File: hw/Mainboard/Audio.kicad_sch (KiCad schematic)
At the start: 10 parts, among them J1 SJ-43504-SMT-TR, J8 SPEAKER, Q2 MMBT3904

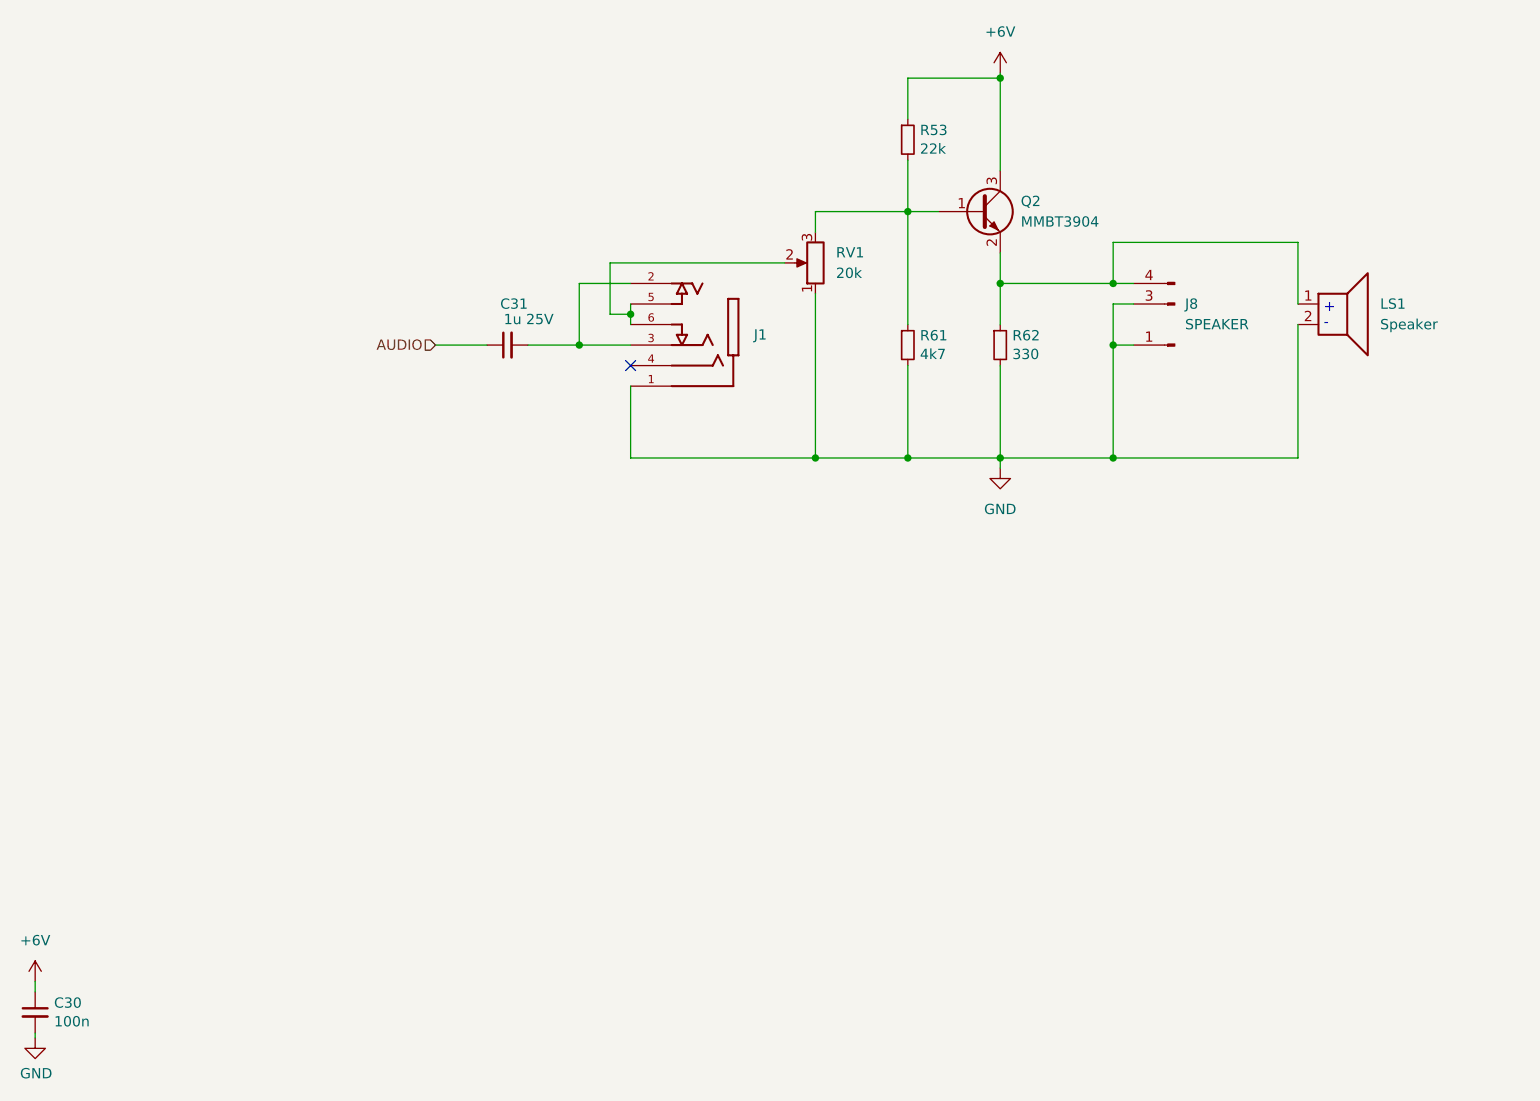
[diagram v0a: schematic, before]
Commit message: hw: wip
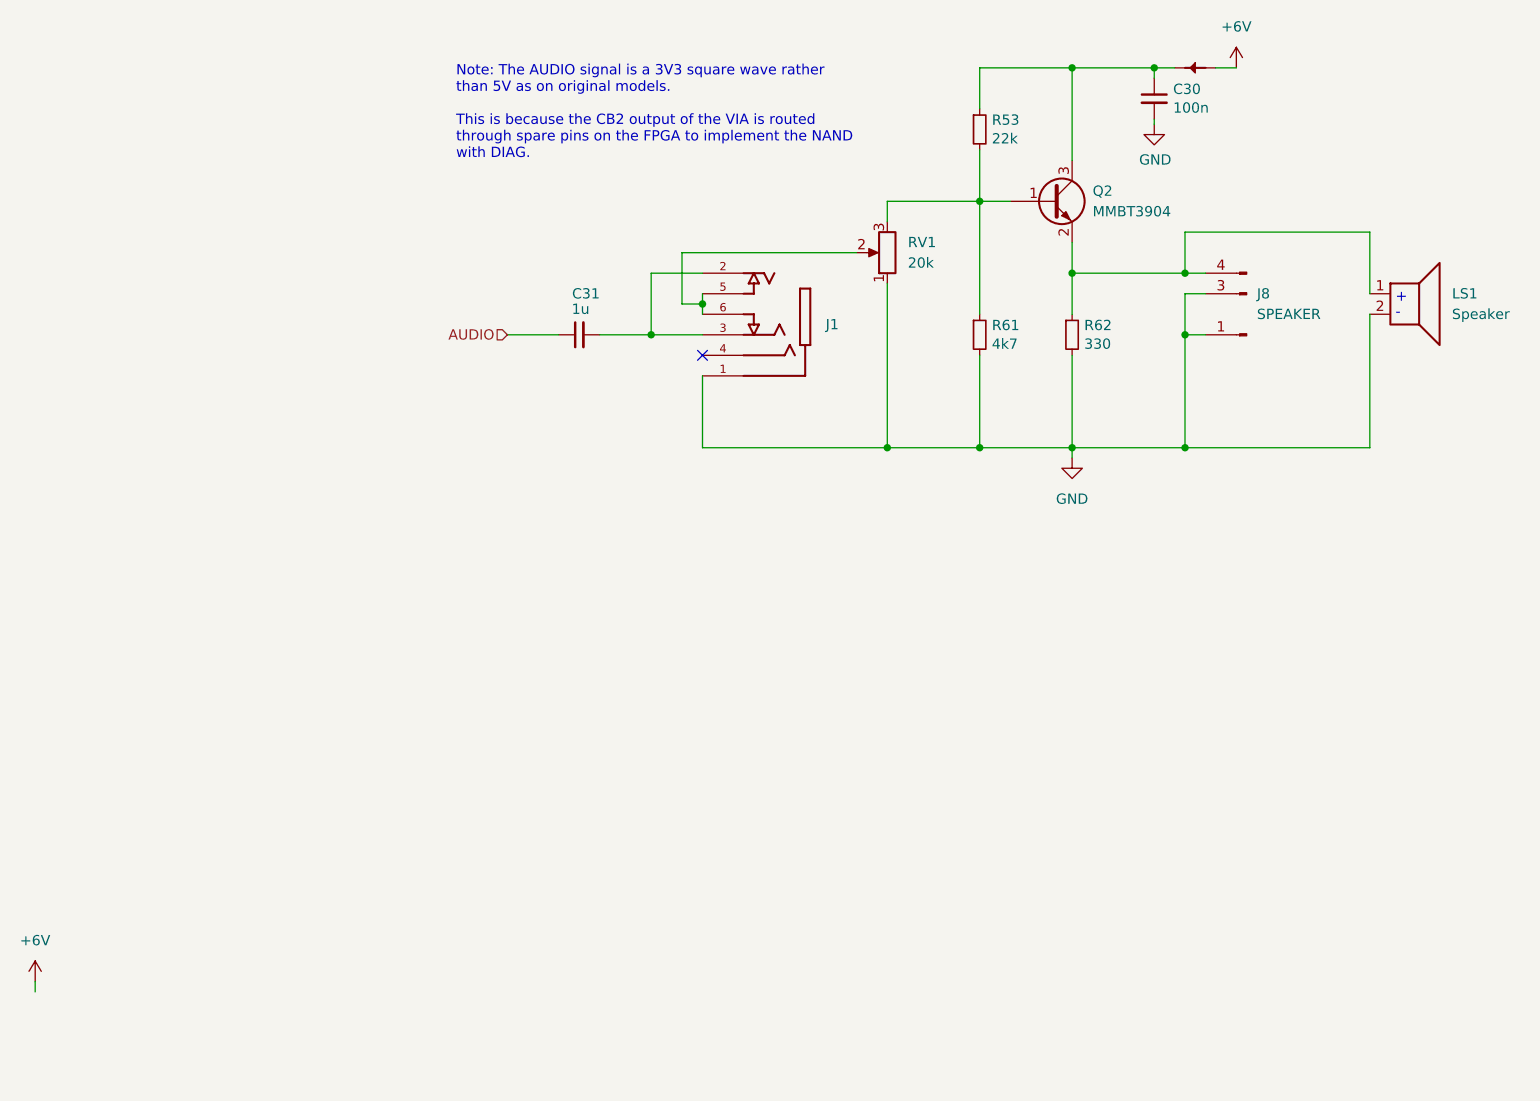
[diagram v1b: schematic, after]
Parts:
- added PT26: PowerTie_2, PET:NetTie-2_SMD_Pad_1.6_to_0.4mm, symbol PET:PowerTie_2
- C31: value 1u 25V -> 1u
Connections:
- net +6V: now also PT26.1; no longer C30.1, Q2.3 (C), R53.1
- new net: C30.1, PT26.2, Q2.3 (C), R53.1
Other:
- note added: "Note: The AUDIO signal is a 3V3 square wave rather than 5V as on original models. This is because the CB2 output of the VIA is routed through spare pins on the FPGA to implement the NAND with DIAG."
- moved on the sheet: C30, C31, J1, J8, LS1, Q2, R53, R61, R62, RV1
